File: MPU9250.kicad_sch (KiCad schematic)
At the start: 19 parts, among them Q6 BSS138, Q7 BSS138, U11 MAX30102, U12 LN1134A182MR-G, U13 MPU-9250

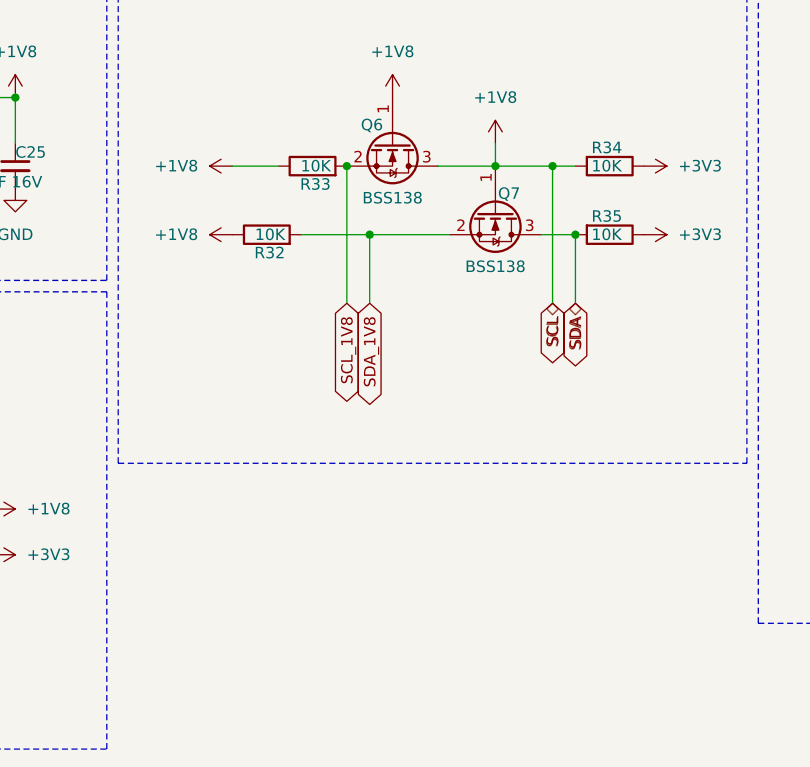
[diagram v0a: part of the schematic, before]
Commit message: Update Board
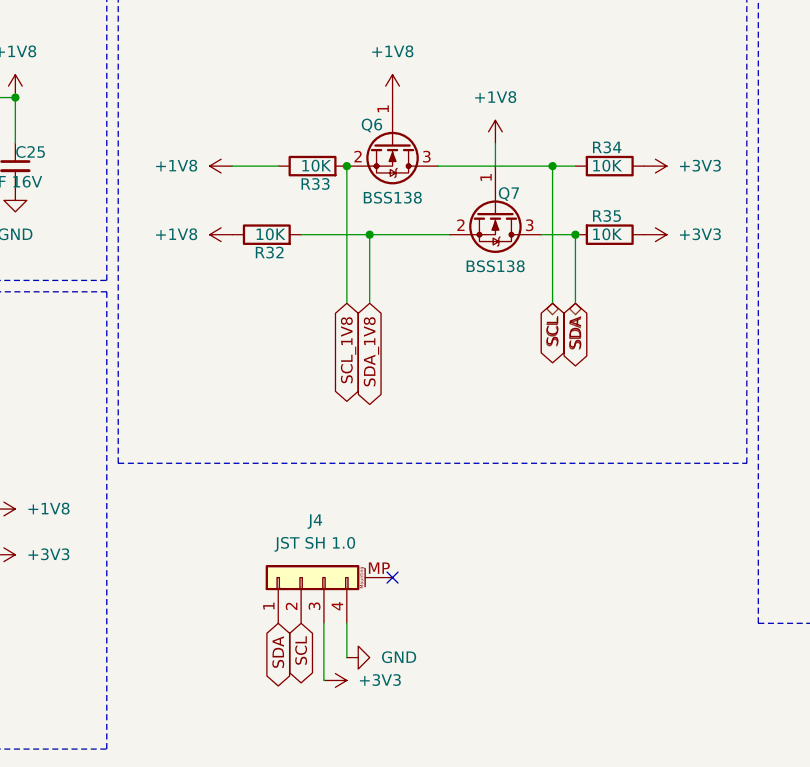
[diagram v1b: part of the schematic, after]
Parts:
- added J4: JST SH 1.0, Connector_JST:JST_SH_SM04B-SRSS-TB_1x04-1MP_P1.00mm_Horizontal, symbol Connector_Generic_MountingPin:Conn_01x04_MountingPin
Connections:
- net +1V8: no longer Q6.3 (D), R34.2, U13.23 (SCL/SCLK)
- net +3V3: now also J4.3 (Pin_3)
- net GND: now also J4.4 (Pin_4)
- net SDA: now also J4.1 (Pin_1)
- new net SCL: J4.2 (Pin_2), Q6.3 (D), R34.2, U13.23 (SCL/SCLK)
- no-connect marks 2 -> 3
